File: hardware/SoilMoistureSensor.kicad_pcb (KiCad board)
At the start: 2 copper layers, 30 parts, among them Q1 AO3401A, SW1 SW_Push, SW2 SW_Push, U1 BQ25570, U2 ESP32-C3-WROOM-02, U3 TLC555xD

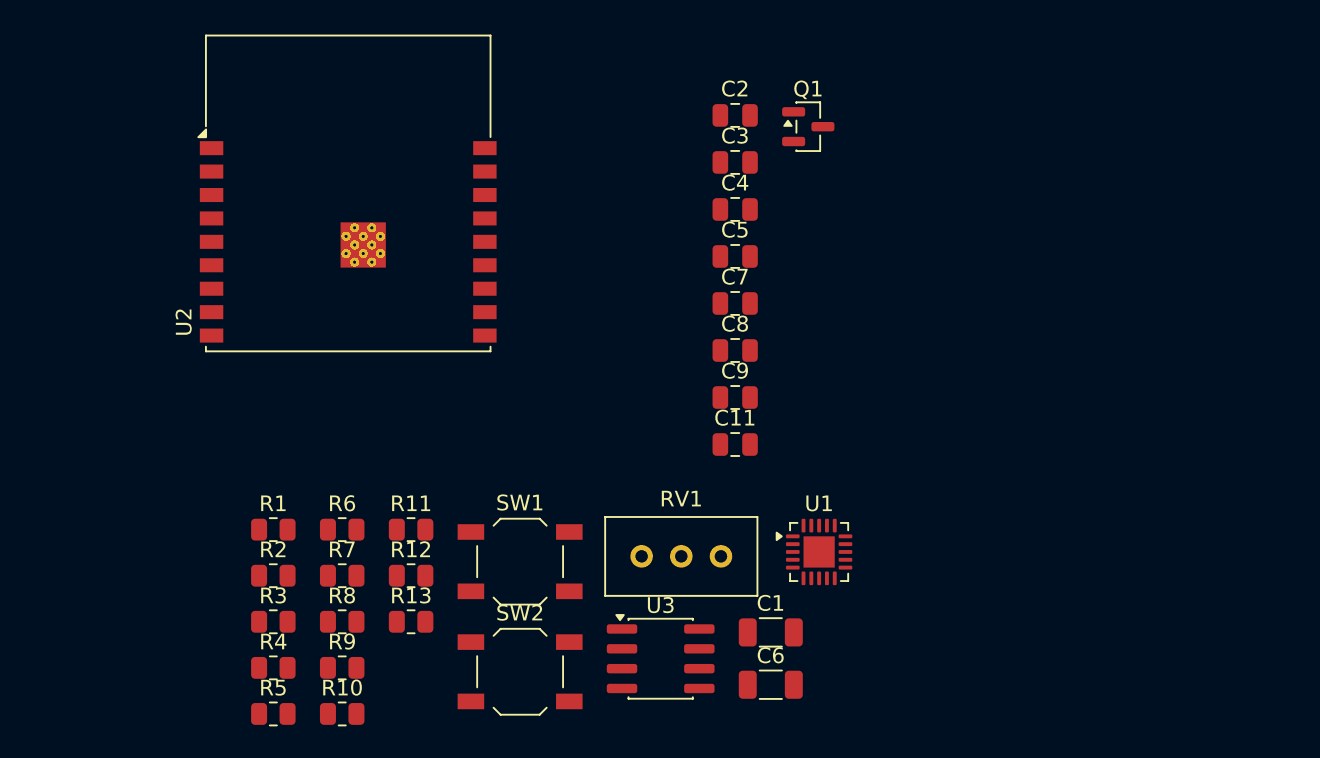
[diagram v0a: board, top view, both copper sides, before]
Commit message: started layout in pcb
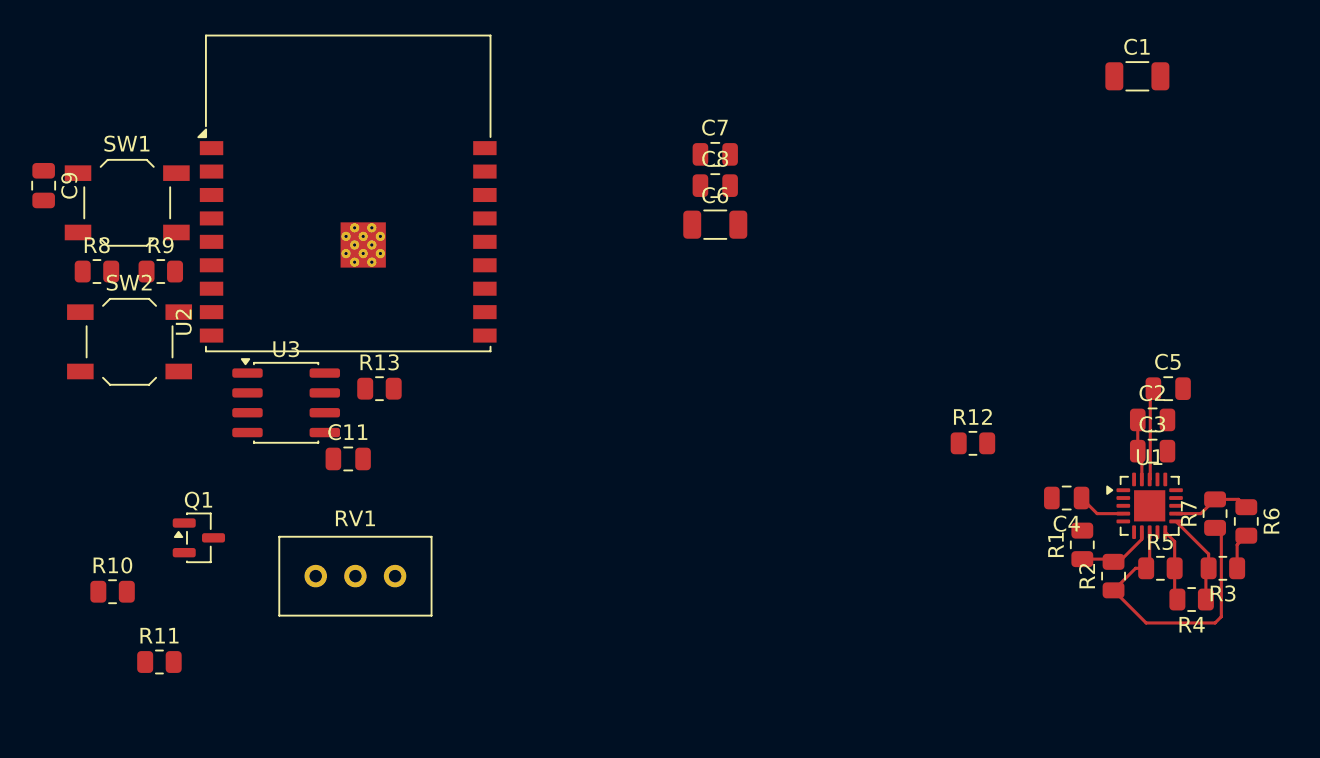
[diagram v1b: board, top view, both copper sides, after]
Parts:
- moved R3 60.9 mm to (172.5, 86.5), turned to 180 degrees
- moved R4 59.0 mm to (170.5, 88.5), turned to 180 degrees
- moved R6 57.9 mm to (174.0, 83.5), turned to -90 degrees
- moved R5 57.6 mm to (168.5, 86.5)
- moved R7 56.0 mm to (172.0, 83.0), turned to 90 degrees
- moved R2 53.8 mm to (165.5, 87.0), turned to 90 degrees
- moved R1 51.8 mm to (163.5, 85.0), turned to 90 degrees
- moved Q1 47.1 mm to (106.9, 84.5)
- moved C9 46.3 mm to (97.0, 62.0), turned to -90 degrees
- moved C1 42.6 mm to (167.0, 55.0)
- moved R12 37.0 mm to (156.5, 78.5)
- moved SW1 34.1 mm to (102.3, 63.1)
- moved C2 33.1 mm to (168.0, 77.0)
- moved SW2 32.7 mm to (102.5, 72.0)
- moved C3 32.5 mm to (168.0, 79.0)
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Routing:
- net /VRDIV: track 0.00 -> 18.9 mm
- net /OK_PROG_N: track 0.00 -> 5.94 mm
- net /VBAT: track 0.00 -> 5.91 mm
- net /VOUT_SET_N: track 0.00 -> 5.09 mm
- net /VBAT_OV_N: track 0.00 -> 4.94 mm
- net /OK_HYST_N: track 0.00 -> 4.63 mm
- net /VSTOR: track 0.00 -> 3.92 mm
- net /VREF_SAMP: track 0.00 -> 3.09 mm
- net GND: track 0.00 -> 2.33 mm
